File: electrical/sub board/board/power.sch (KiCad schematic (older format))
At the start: 31 parts, among them U301 RT7263A, U302 RT7263A, U303 RT7263A

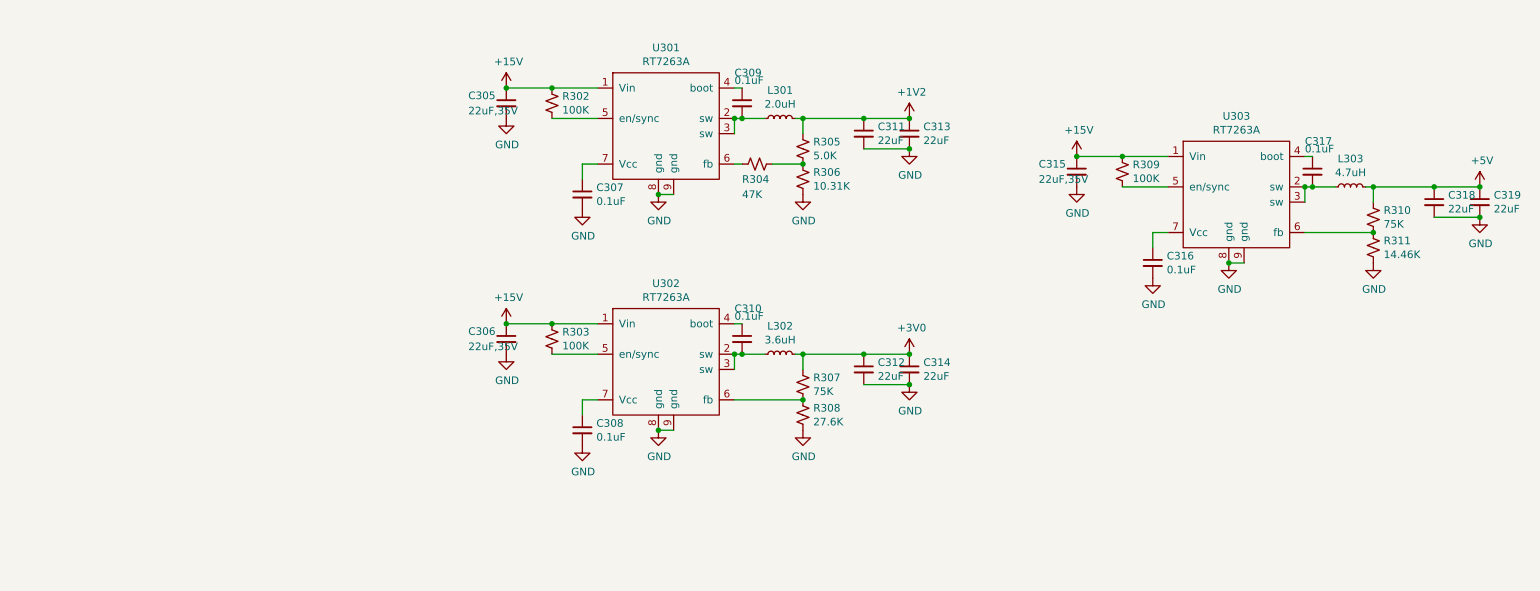
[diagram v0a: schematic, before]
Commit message: updated sub board
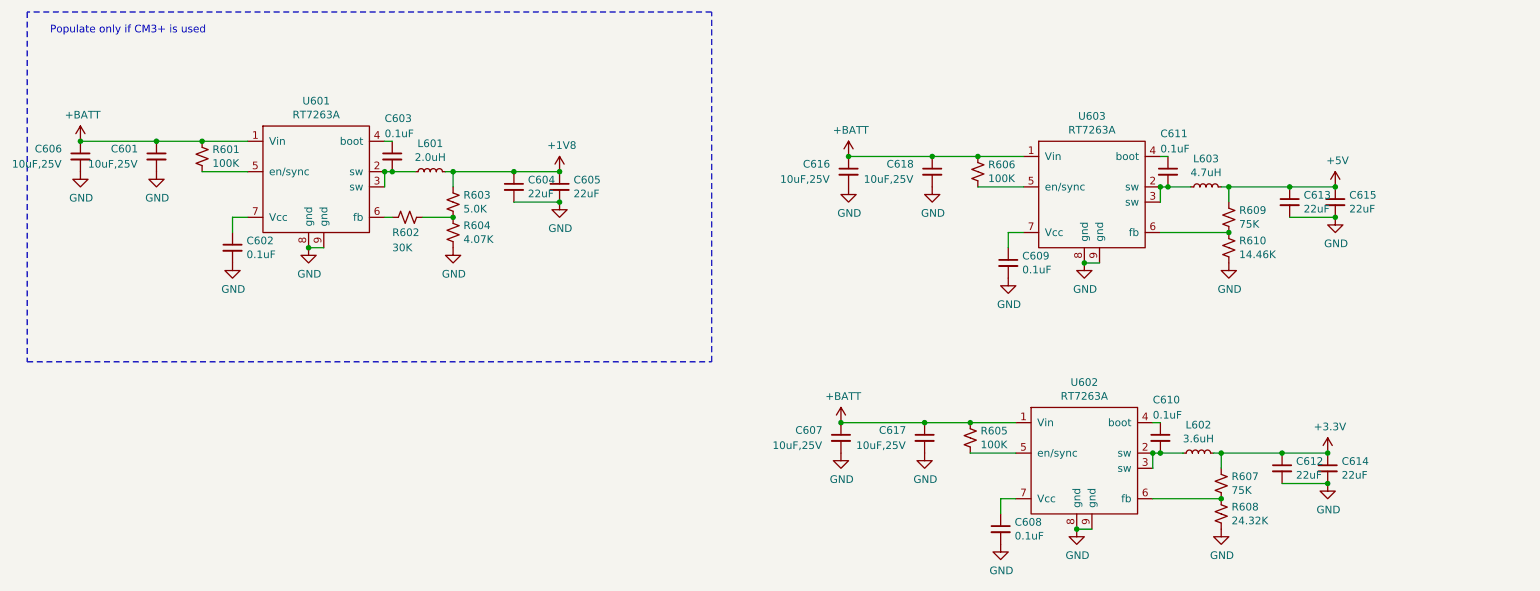
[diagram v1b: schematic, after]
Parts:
- removed C306, C315: 22uF,35V, Capacitor_SMD:C_1210_3225Metric, symbol Device:C_Small
- added C606, C607, C616, C617, C618: 10uF,25V, Capacitor_SMD:C_1206_3216Metric, symbol Device:C_Small
- C601: renamed from C305; value 22uF,35V -> 10uF,25V; footprint Capacitor_SMD:C_1210_3225Metric -> Capacitor_SMD:C_1206_3216Metric
- L601: renamed from L301; footprint holo:NR8040 -> sub:NR8040
- L602: renamed from L302; footprint holo:NR8040 -> sub:NR8040
- L603: renamed from L303; footprint holo:NR8040 -> sub:NR8040
- R602: renamed from R304; value 47K -> 30K
- R604: renamed from R306; value 10.31K -> 4.07K
- R608: renamed from R308; value 27.6K -> 24.32K
- U601: renamed from U301; footprint holo:SOP-EP-8_3.9x4.9mm_P1.27mm -> sub:SOP-EP-8_3.9x4.9mm_P1.27mm
- U602: renamed from U302; footprint holo:SOP-EP-8_3.9x4.9mm_P1.27mm -> sub:SOP-EP-8_3.9x4.9mm_P1.27mm
- U603: renamed from U303; footprint holo:SOP-EP-8_3.9x4.9mm_P1.27mm -> sub:SOP-EP-8_3.9x4.9mm_P1.27mm
- renumbered C307 to C602, C309 to C603, C311 to C604, C313 to C605, C308 to C608, C316 to C609, C310 to C610, C317 to C611, C312 to C612, C318 to C613, C314 to C614, C319 to C615, R302 to R601, R305 to R603, R303 to R605, R309 to R606, R307 to R607, R310 to R609, R311 to R610
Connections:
- net GND: now also C606.2, C607.2, C616.2, C617.2, C618.2
- net +15V renamed +BATT
- net +BATT: now also C606.1, C607.1, C616.1, C617.1, C618.1
- net +1V2 renamed +1V8
- net +3V0 renamed +3V3
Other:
- note added: "Populate only if CM3+ is used"
- moved on the sheet: C601, C602, C603, C604, C605, C608, C609, C610, C611, C612, C613, C614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
